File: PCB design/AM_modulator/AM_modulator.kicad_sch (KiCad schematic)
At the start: 4 parts, among them J1 AudioJack3, J2 Conn_01x02_Female, SW1 SW_DIP_x01, SW2 SW_DIP_x01

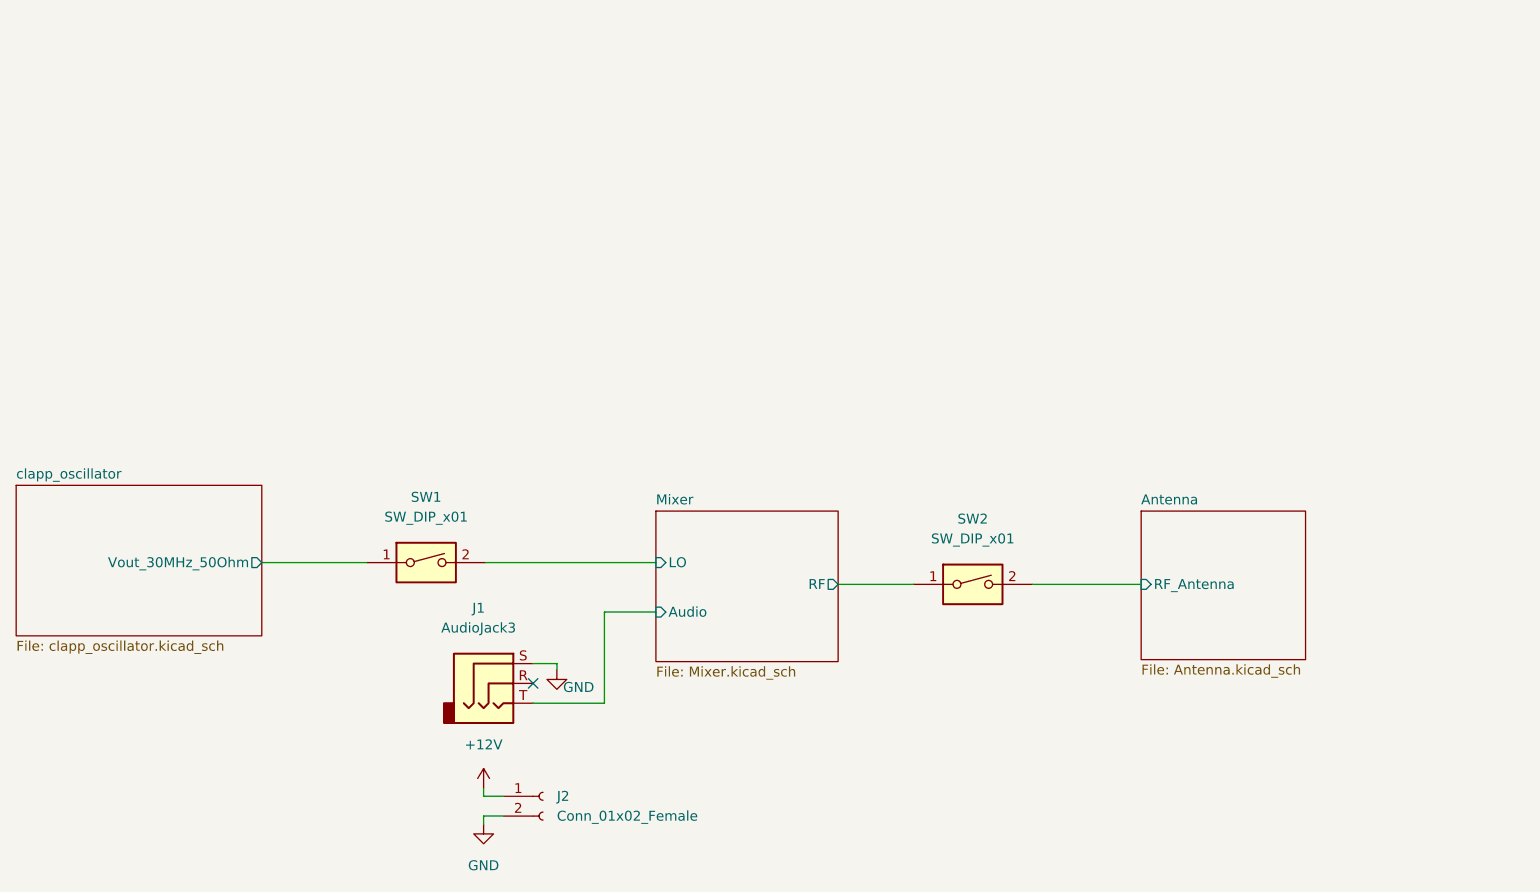
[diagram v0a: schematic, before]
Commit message: PCB design done
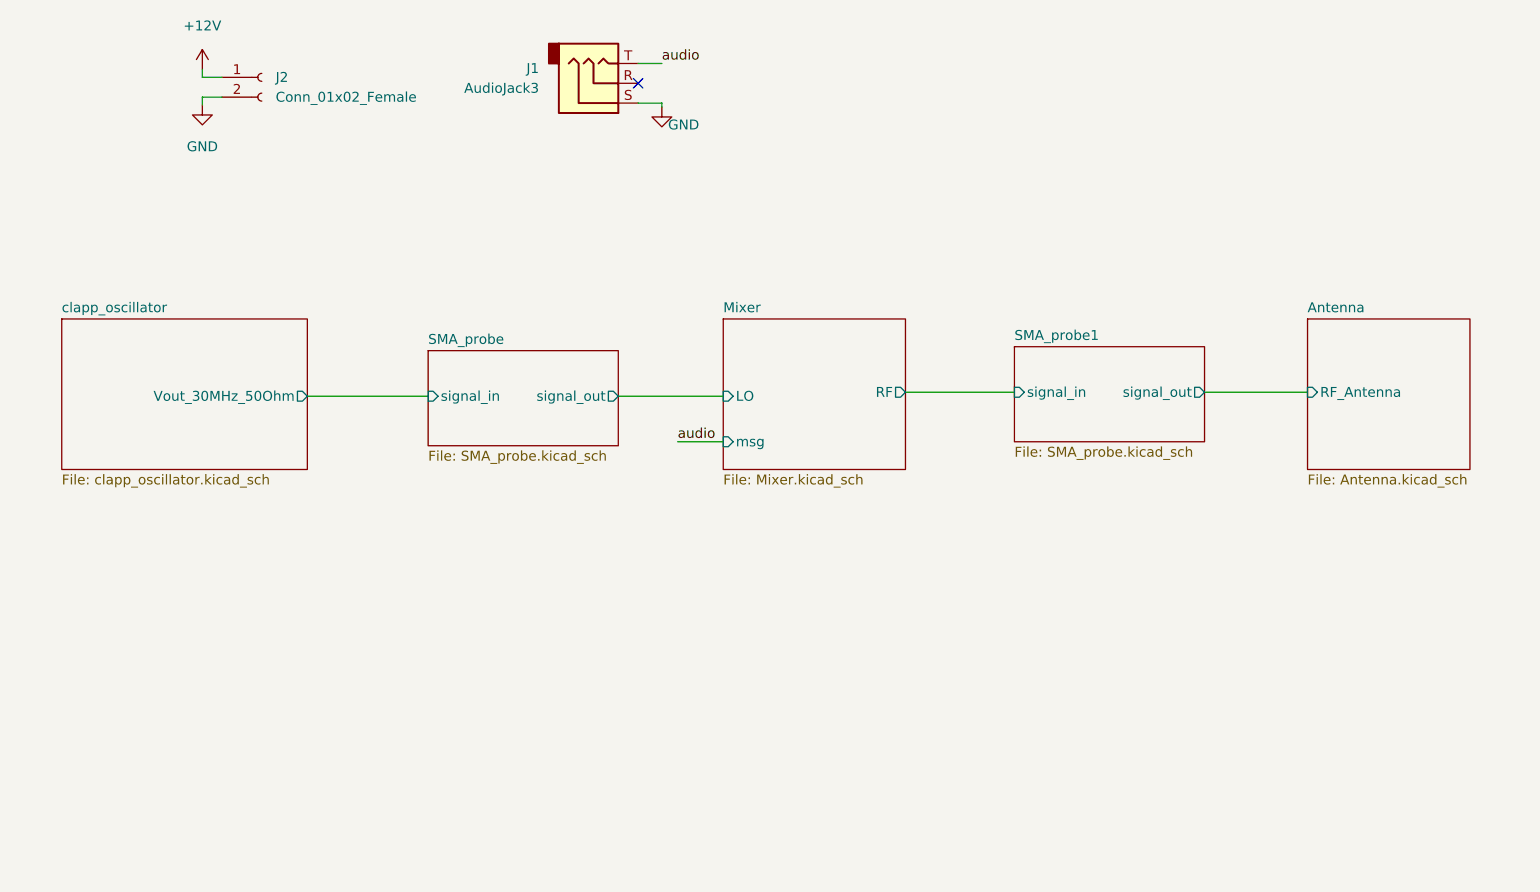
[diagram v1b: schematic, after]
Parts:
- removed SW1, SW2: SW_DIP_x01, Resistor_SMD:R_0603_1608Metric_Pad0.98x0.95mm_HandSolder, symbol Switch:SW_DIP_x01
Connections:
- net Mixer/Audio renamed audio
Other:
- added sheet SMA_probe (SMA_probe.kicad_sch)
- added sheet SMA_probe1 (SMA_probe.kicad_sch)
- sheet Mixer ports: added msg; removed Audio
- moved on the sheet: J1, J2
